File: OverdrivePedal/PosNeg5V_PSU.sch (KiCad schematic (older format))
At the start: 17 parts, among them U2 TC7662Bx0A, U3 MIC5233YM5, U4 MIC5270YM5

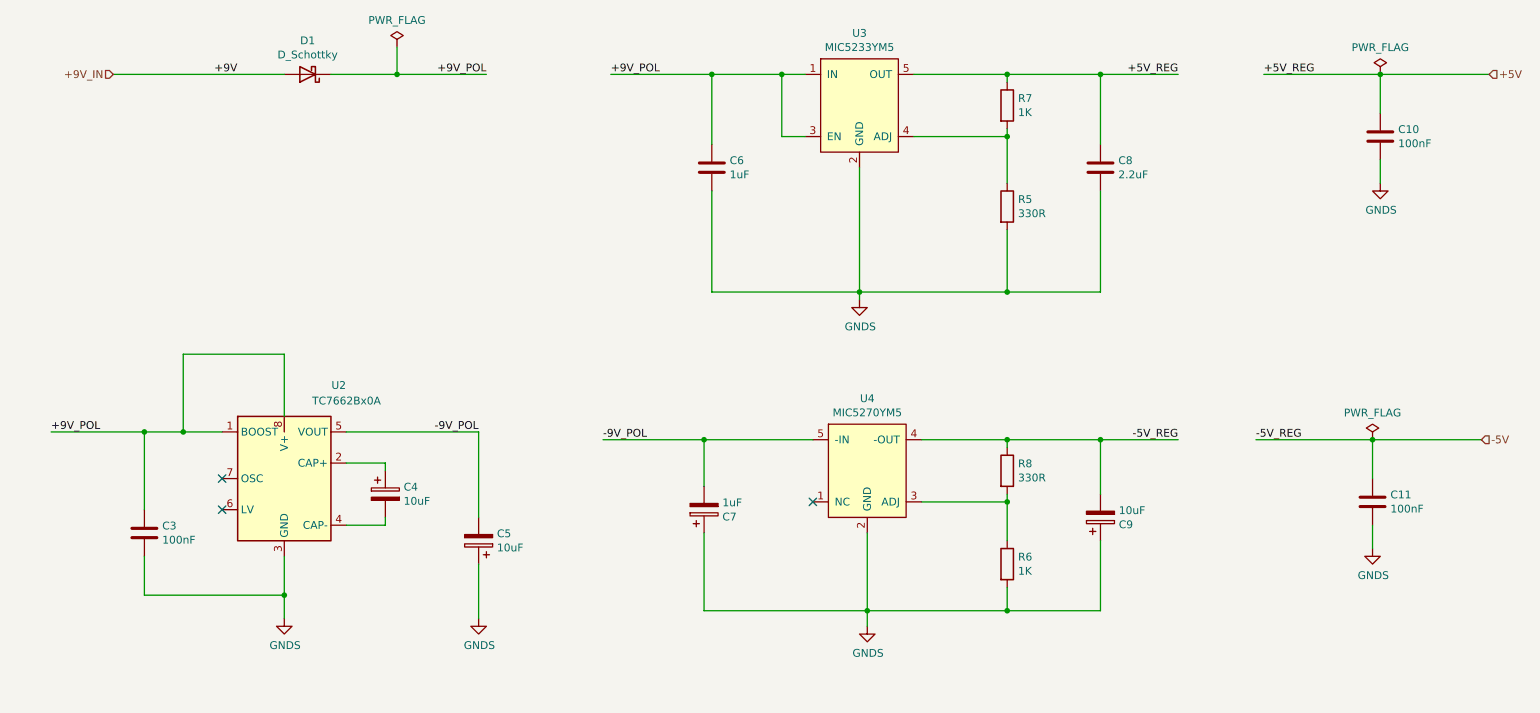
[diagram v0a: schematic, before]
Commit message: updates
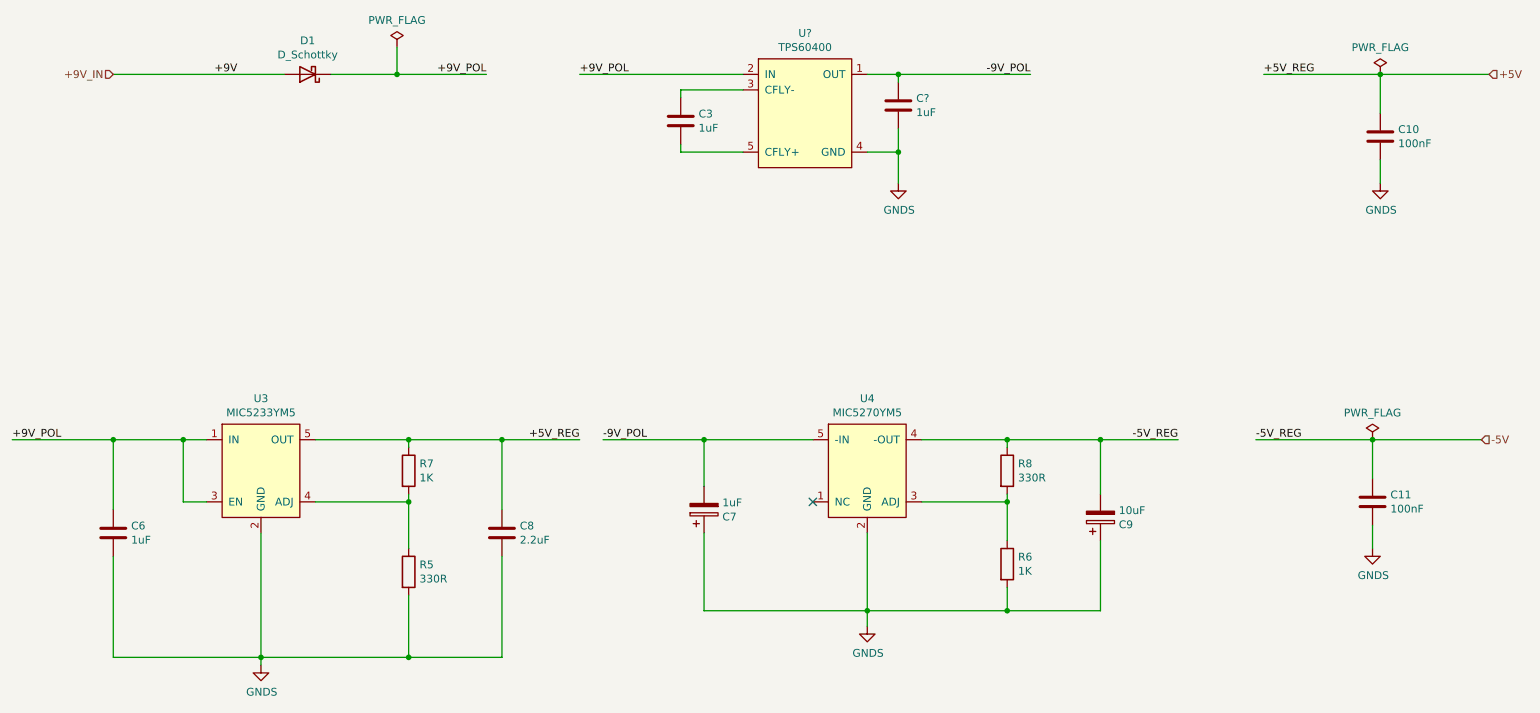
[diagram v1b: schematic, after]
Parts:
- removed C4, C5: 10uF, Capacitor_SMD:CP_Elec_4x5.7, symbol Device:CP
- removed U2: TC7662Bx0A, Package_SO:SOIC-8_3.9x4.9mm_P1.27mm, symbol OverdrivePedal-rescue:TC7662Bx0A-Converter_DCDC
- added C?: 1uF, Capacitor_SMD:C_0805_2012Metric_Pad1.15x1.40mm_HandSolder, symbol Device:C
- added U?: TPS60400, Package_TO_SOT_SMD:SOT-23-5_HandSoldering, symbol TPS6040x:TPS60400
- C3: value 100nF -> 1uF
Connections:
- net +9V_POL: now also U?.2 (IN); no longer C3.1
- net -9V_POL: now also C?.1, U?.1 (OUT)
- net GNDS: now also C?.2, U?.4 (GND); no longer C3.2
- new net: C3.1, U?.3 (CFLY-)
- new net: C3.2, U?.5 (CFLY+)
- no-connect marks 3 -> 1
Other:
- moved on the sheet: C3, C6, C8, R5, R7, U3
